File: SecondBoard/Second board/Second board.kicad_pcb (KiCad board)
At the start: 2 copper layers, 5 parts

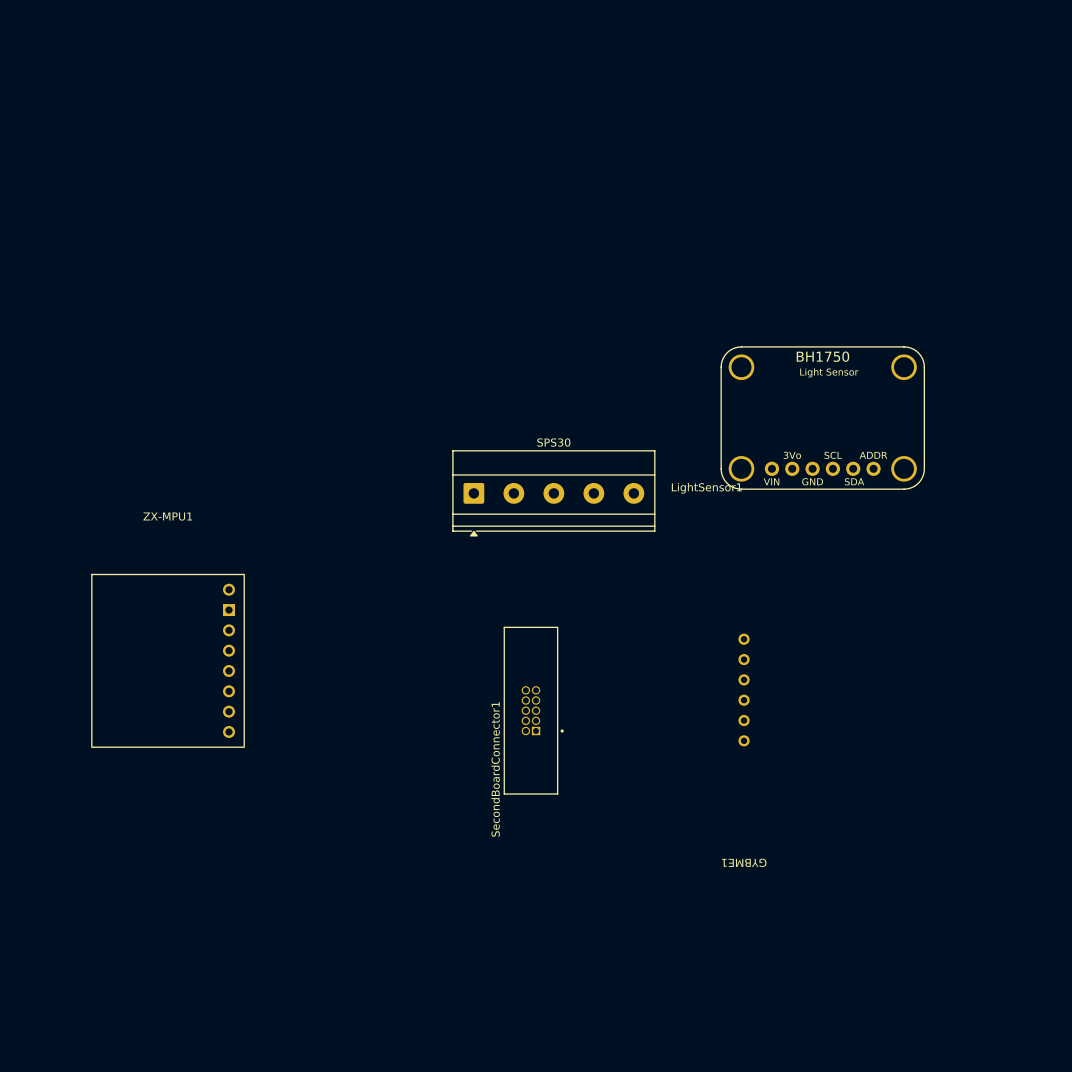
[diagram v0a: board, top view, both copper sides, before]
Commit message: SecondBoard Rond m130
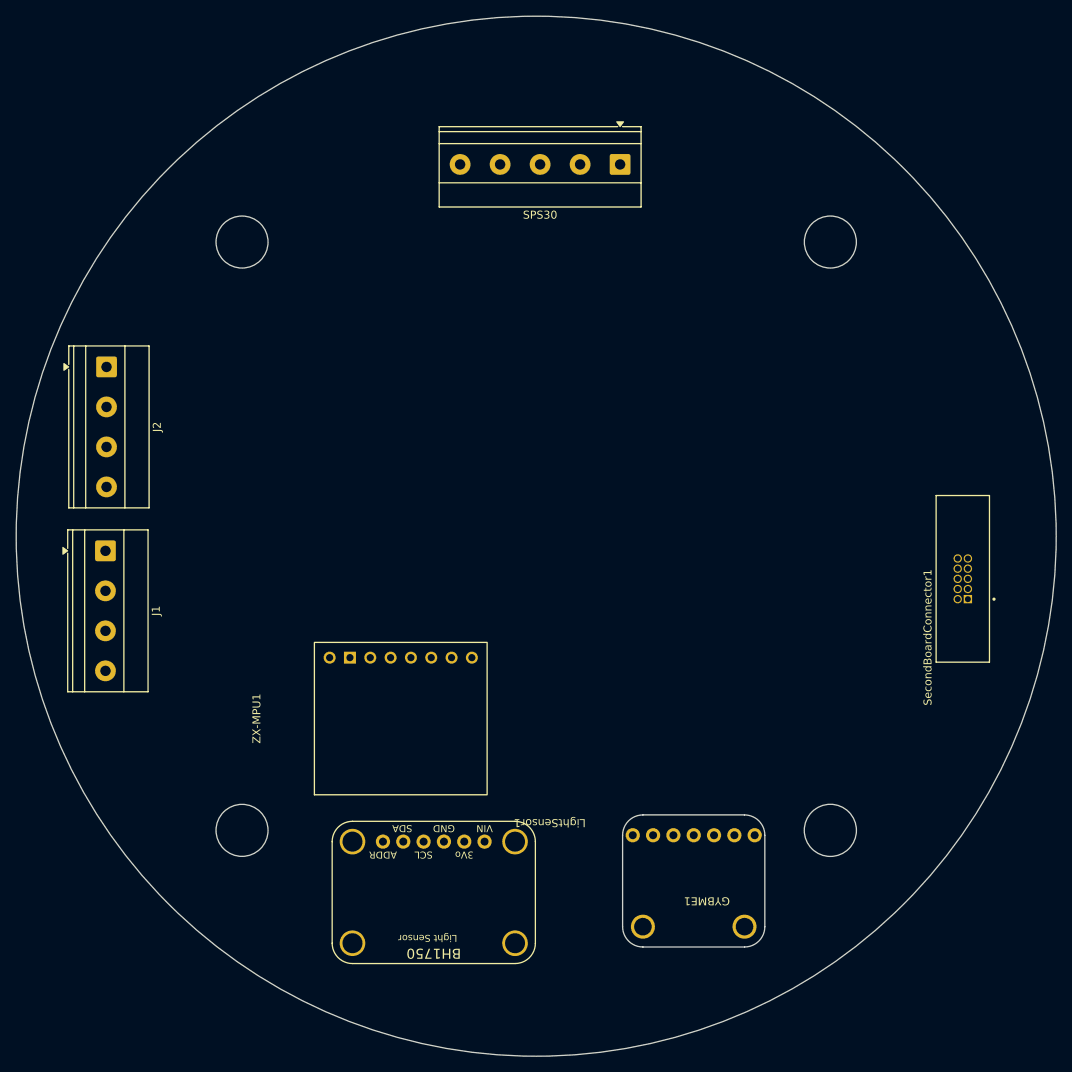
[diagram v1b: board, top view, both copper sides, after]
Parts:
- added J1: Conn_01x04_Socket, TerminalBlock_Phoenix:TerminalBlock_Phoenix_MKDS-1,5-4_1x04_P5.00mm_Horizontal, F.Cu at (93.7, 93.2)
- added J2: Conn_01x04_Socket, TerminalBlock_Phoenix:TerminalBlock_Phoenix_MKDS-1,5-4_1x04_P5.00mm_Horizontal, F.Cu at (93.8, 70.3)
- GYBME1: footprint custom footprints:GY-BME280_P -> custom footprints:Sans titre
- moved SecondBoardConnector1 56.4 mm to (200.8, 96.8)
- moved LightSensor1 45.4 mm to (149.2, 126.8), turned to 180 degrees
- moved SPS30 45.0 mm to (158.0, 44.9), turned to 180 degrees
- moved ZX-MPU1 31.7 mm to (139.5, 106.6), turned to 90 degrees
- moved GYBME1 17.3 mm to (177.0, 133.9)
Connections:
- GYBME1 pad 3: Net-(GYBME1-SCL) -> unconnected-(GYBME1-GND-Pad3)
- GYBME1 pad 4: Net-(GYBME1-SDA) -> Net-(GYBME1-SCK)
- GYBME1 pad 6: unconnected-(GYBME1-SDO-Pad6) -> Net-(GYBME1-SDI)
- LightSensor1 pad 4: Net-(GYBME1-SCL) -> Net-(GYBME1-SCK)
- LightSensor1 pad 5: Net-(GYBME1-SDA) -> Net-(GYBME1-SDI)
- SPS30 pad 2: Net-(GYBME1-SDA) -> Net-(GYBME1-SDI)
- SPS30 pad 3: Net-(GYBME1-SCL) -> Net-(GYBME1-SCK)
- SecondBoardConnector1 pad 10: Net-(GYBME1-SDA) -> Net-(GYBME1-SDI)
- SecondBoardConnector1 pad 8: Net-(GYBME1-SCL) -> Net-(GYBME1-SCK)
- ZX-MPU1 pad 3: Net-(GYBME1-SCL) -> Net-(GYBME1-SCK)
- ZX-MPU1 pad 4: Net-(GYBME1-SDA) -> Net-(GYBME1-SDI)
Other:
- board outline added: 130 x 130 mm
